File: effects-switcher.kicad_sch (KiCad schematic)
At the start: 56 parts, among them J1 In, J10 L4-In, J11 L4-Out, J12 Conn_01x02, J2 Out, J3 Tuner, J34 Conn_01x02, J4 L1-In, J5 L1-Out, J56 Conn_01x02, J6 L2-In, J7 L2-Out, J8 L3-In, J9 L3-Out, K1 Bypass, K2 Tuner, K3 Loop1, K4 Loop2, K5 Loop3, K6 Loop4, Q1 2N3904, Q2 2N3904, Q3 2N3904, Q4 2N3904, Q5 2N3904, Q6 2N3904, U1 LM7805

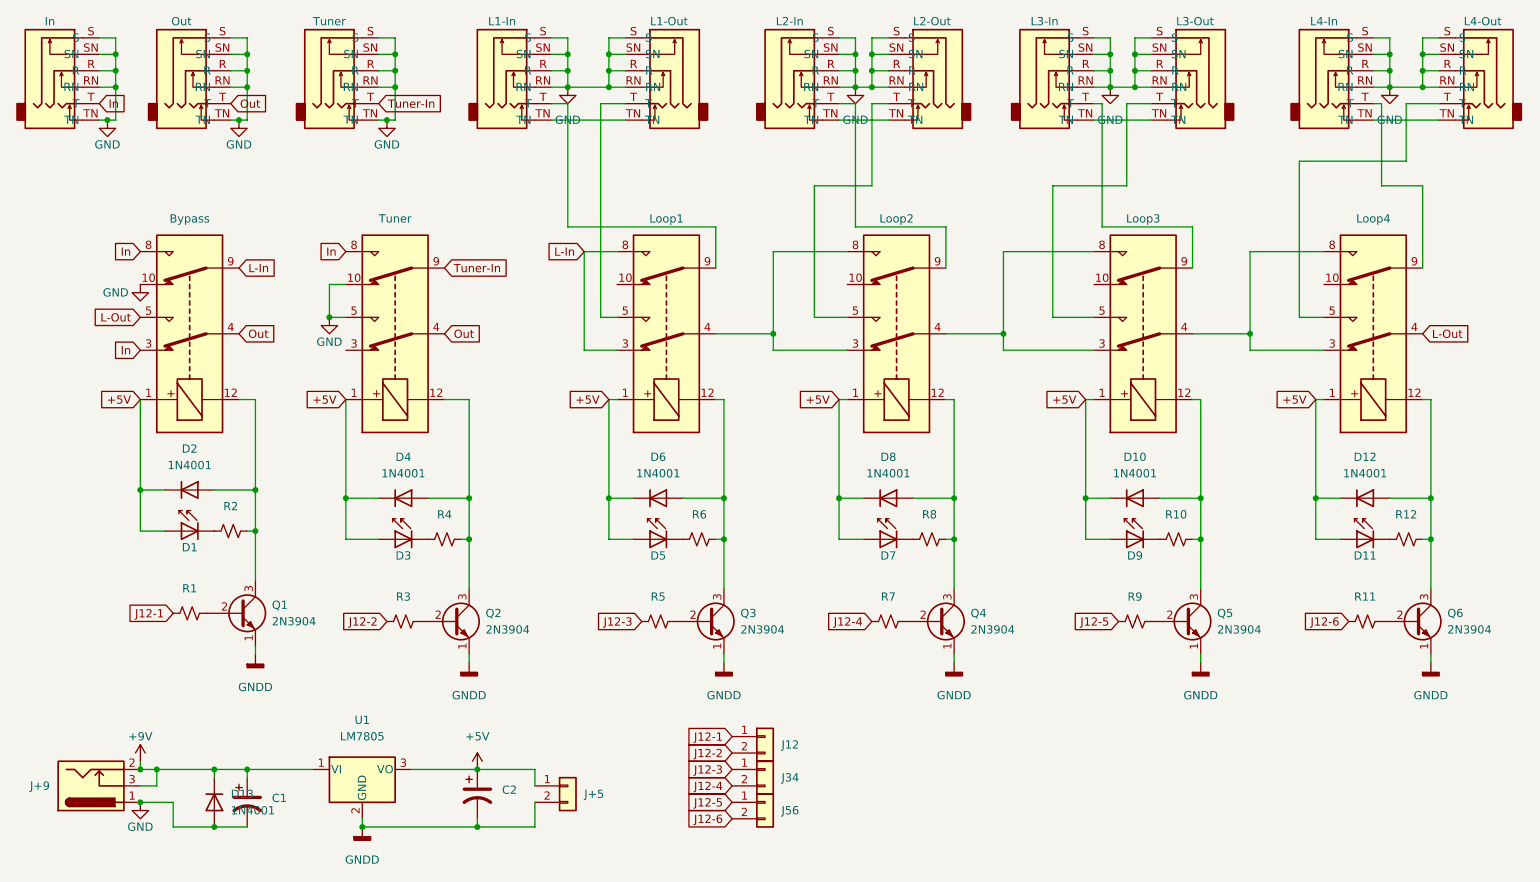
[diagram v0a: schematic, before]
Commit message: Revert "removed 9v out"
This reverts commit 68eda4370ce2c703412f077e884cf7a60c7e0849.
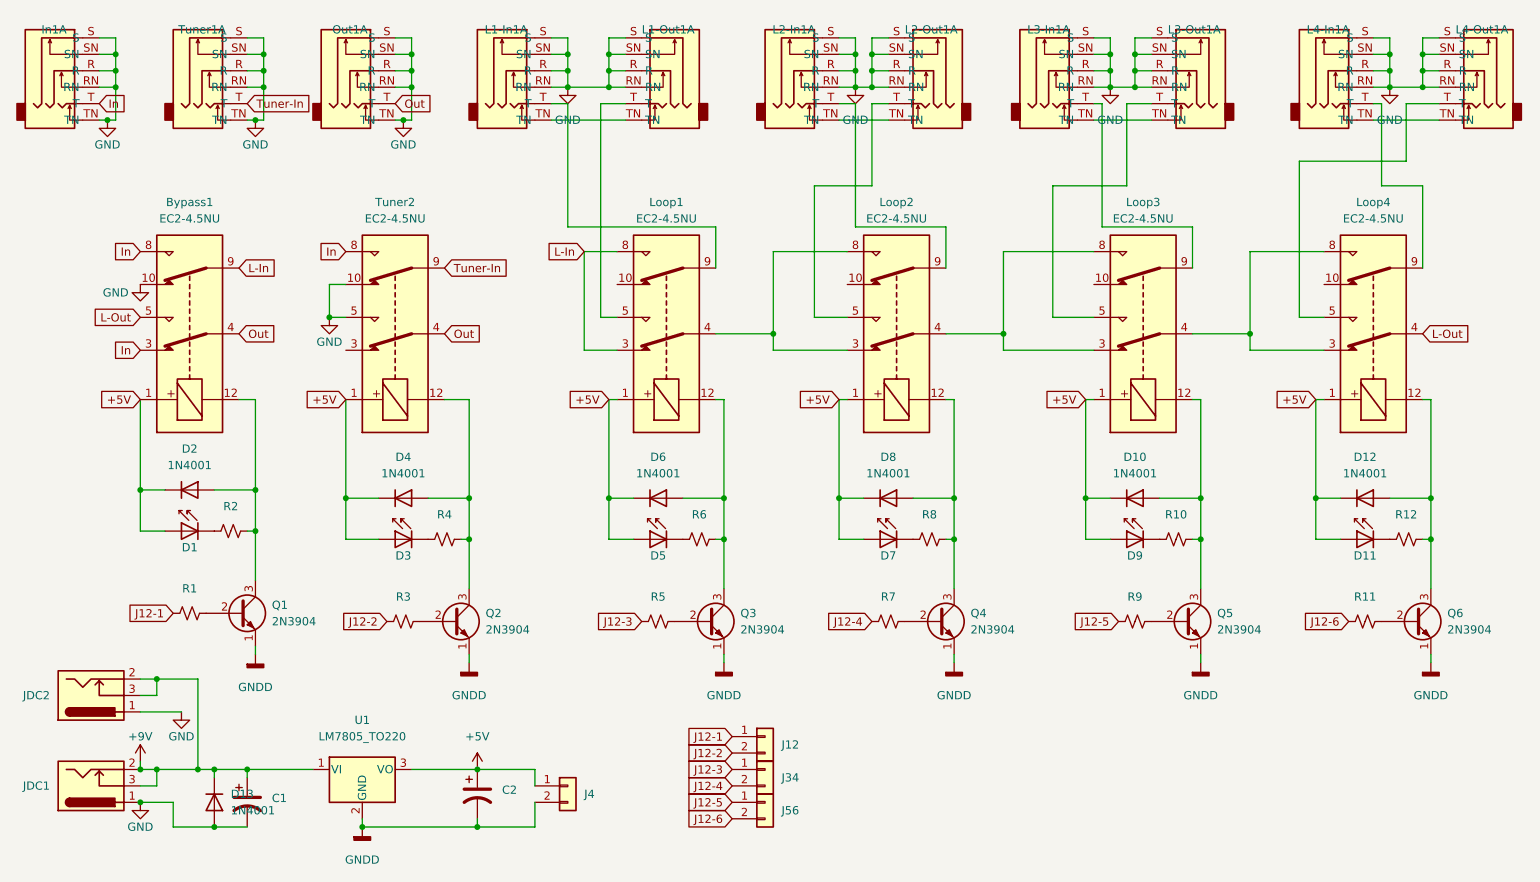
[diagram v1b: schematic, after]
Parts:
- added JDC2: Barrel_Jack_Switch, Connector_BarrelJack:BarrelJack_Horizontal, symbol Connector:Barrel_Jack_Switch
- Bypass1: renamed from K1; value Bypass -> EC2-4.5NU
- In1: renamed from J1; value In -> AudioJack3_SwitchSTR
- L1-In1: renamed from J4; value L1-In -> AudioJack3_SwitchSTR
- L1-Out1: renamed from J5; value L1-Out -> AudioJack3_SwitchSTR
- L2-In1: renamed from J6; value L2-In -> AudioJack3_SwitchSTR
- L2-Out1: renamed from J7; value L2-Out -> AudioJack3_SwitchSTR
- L3-In1: renamed from J8; value L3-In -> AudioJack3_SwitchSTR
- L3-Out1: renamed from J9; value L3-Out -> AudioJack3_SwitchSTR
- L4-In1: renamed from J10; value L4-In -> AudioJack3_SwitchSTR
- L4-Out1: renamed from J11; value L4-Out -> AudioJack3_SwitchSTR
- Loop1: renamed from K3; value Loop1 -> EC2-4.5NU
- Loop2: renamed from K4; value Loop2 -> EC2-4.5NU
- Loop3: renamed from K5; value Loop3 -> EC2-4.5NU
- Loop4: renamed from K6; value Loop4 -> EC2-4.5NU
- Out1: renamed from J2; value Out -> AudioJack3_SwitchSTR
- Tuner1: renamed from J3; value Tuner -> AudioJack3_SwitchSTR
- Tuner2: renamed from K2; value Tuner -> EC2-4.5NU
- U1: value LM7805 -> LM7805_TO220
- renumbered J+5 to J4, J+9 to JDC1
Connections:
- net +9V: now also JDC2.2, JDC2.3
- net GND: now also JDC2.1

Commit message: removed 9v out
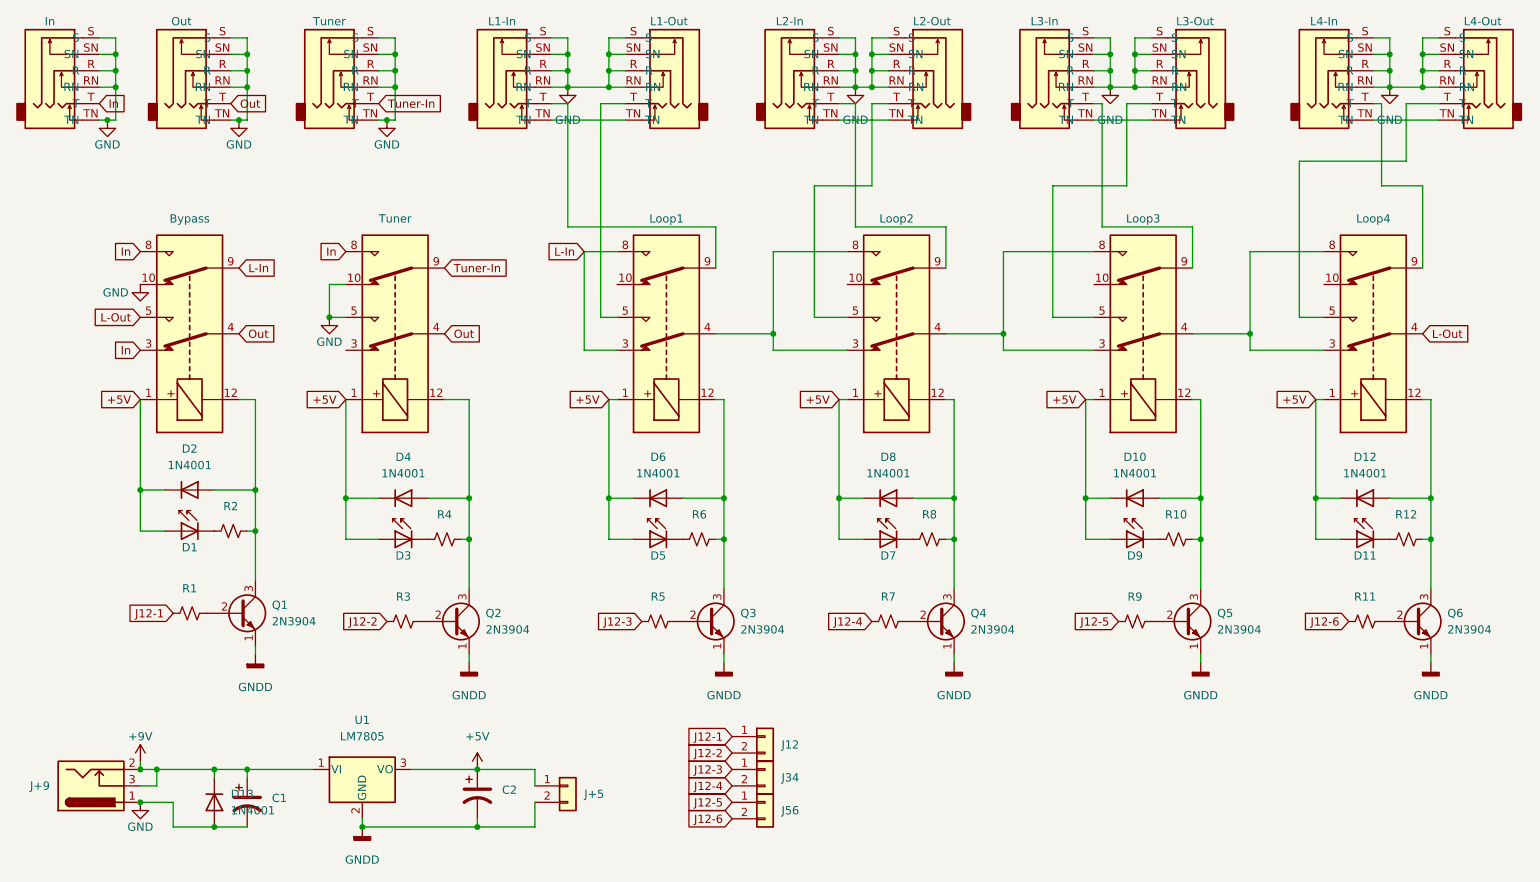
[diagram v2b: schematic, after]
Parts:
- removed JDC2: Barrel_Jack_Switch, Connector_BarrelJack:BarrelJack_Horizontal, symbol Connector:Barrel_Jack_Switch
- J1: renamed from In1; value AudioJack3_SwitchSTR -> In
- J10: renamed from L4-In1; value AudioJack3_SwitchSTR -> L4-In
- J11: renamed from L4-Out1; value AudioJack3_SwitchSTR -> L4-Out
- J2: renamed from Out1; value AudioJack3_SwitchSTR -> Out
- J3: renamed from Tuner1; value AudioJack3_SwitchSTR -> Tuner
- J4: renamed from L1-In1; value AudioJack3_SwitchSTR -> L1-In
- J5: renamed from L1-Out1; value AudioJack3_SwitchSTR -> L1-Out
- J6: renamed from L2-In1; value AudioJack3_SwitchSTR -> L2-In
- J7: renamed from L2-Out1; value AudioJack3_SwitchSTR -> L2-Out
- J8: renamed from L3-In1; value AudioJack3_SwitchSTR -> L3-In
- J9: renamed from L3-Out1; value AudioJack3_SwitchSTR -> L3-Out
- K1: renamed from Bypass1; value EC2-4.5NU -> Bypass
- K2: renamed from Tuner2; value EC2-4.5NU -> Tuner
- K3: renamed from Loop1; value EC2-4.5NU -> Loop1
- K4: renamed from Loop2; value EC2-4.5NU -> Loop2
- K5: renamed from Loop3; value EC2-4.5NU -> Loop3
- K6: renamed from Loop4; value EC2-4.5NU -> Loop4
- U1: value LM7805_TO220 -> LM7805
- renumbered J4 to J+5, JDC1 to J+9
